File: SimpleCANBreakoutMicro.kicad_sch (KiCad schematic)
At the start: 16 parts, among them J1 Conn_01x04_Pin, J2 Conn_01x04_Pin, U2 XC6206PxxxMR, U3 SN65HVD230

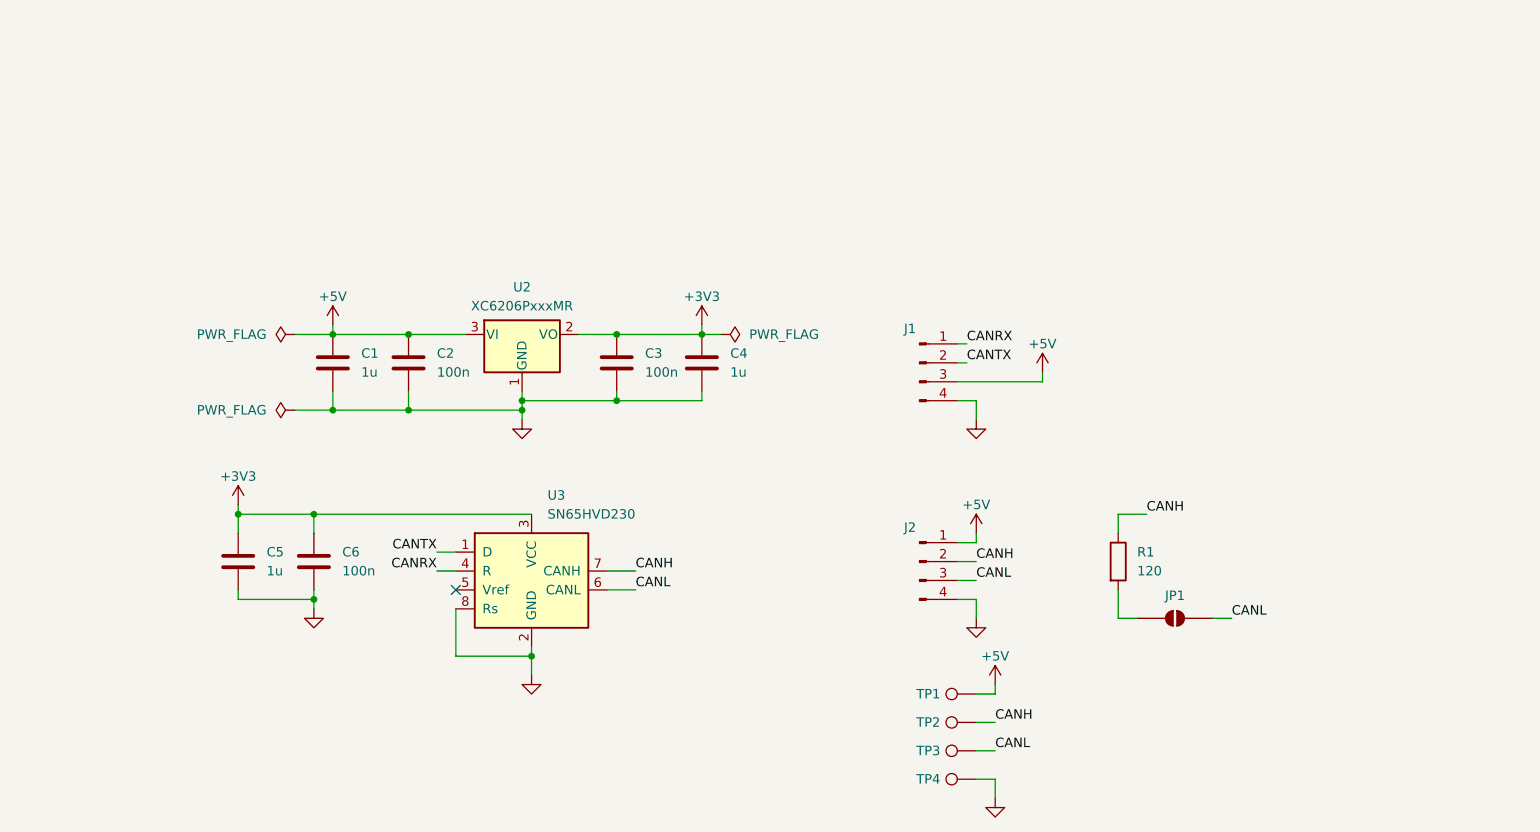
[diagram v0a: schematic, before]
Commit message: Add Schematic
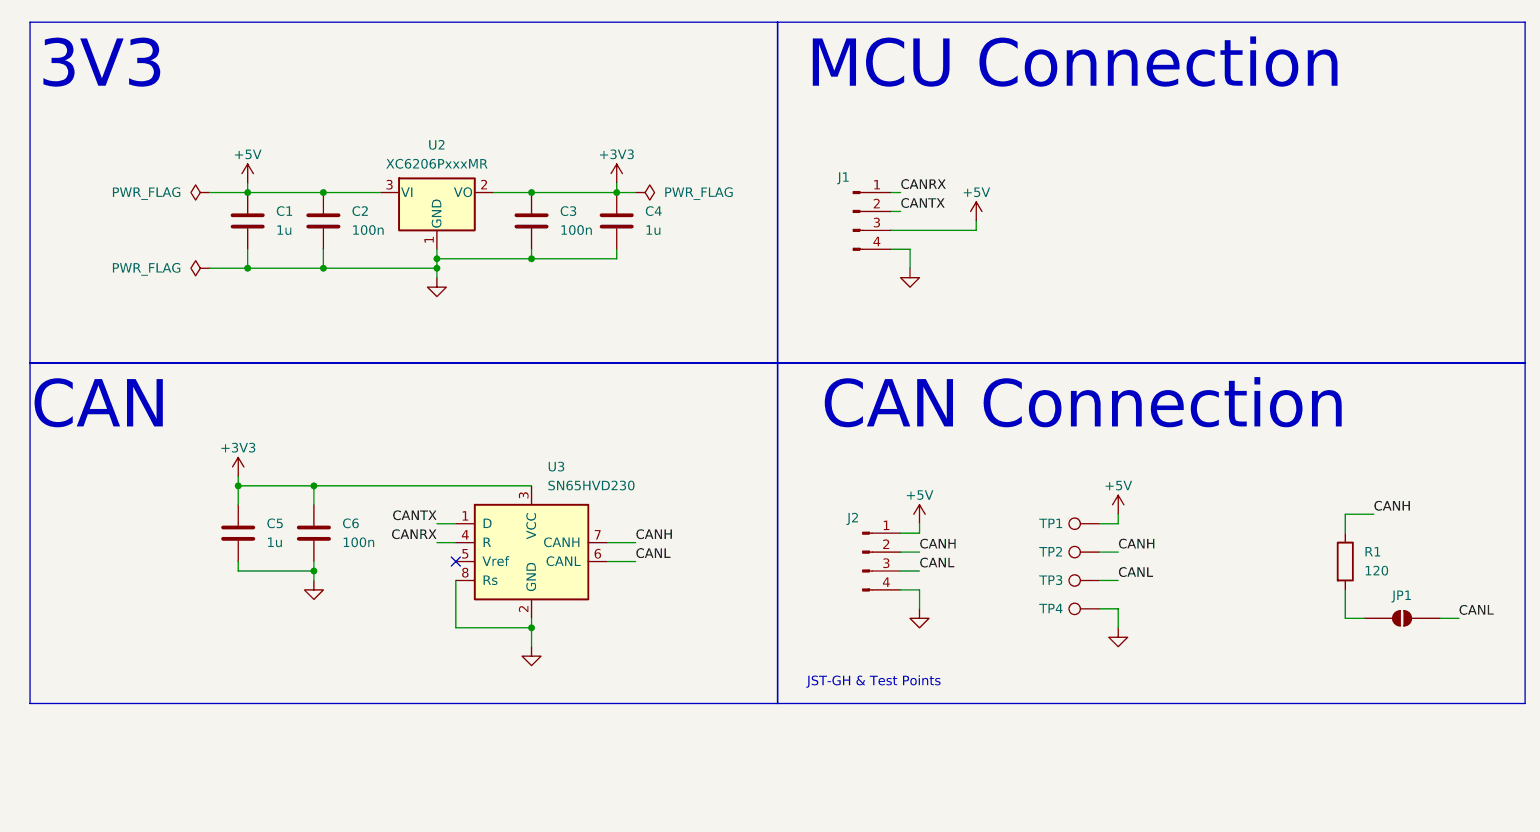
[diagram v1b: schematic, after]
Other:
- note added: "3V3"
- note added: "CAN"
- note added: "CAN Connection"
- note added: "JST-GH & Test Points"
- note added: "MCU Connection"
- moved on the sheet: C1, C2, C3, C4, C5, C6, J1, J2, JP1, R1, TP1, TP2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
